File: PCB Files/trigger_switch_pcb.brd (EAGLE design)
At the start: 114 x 77.5 mm, 11 parts

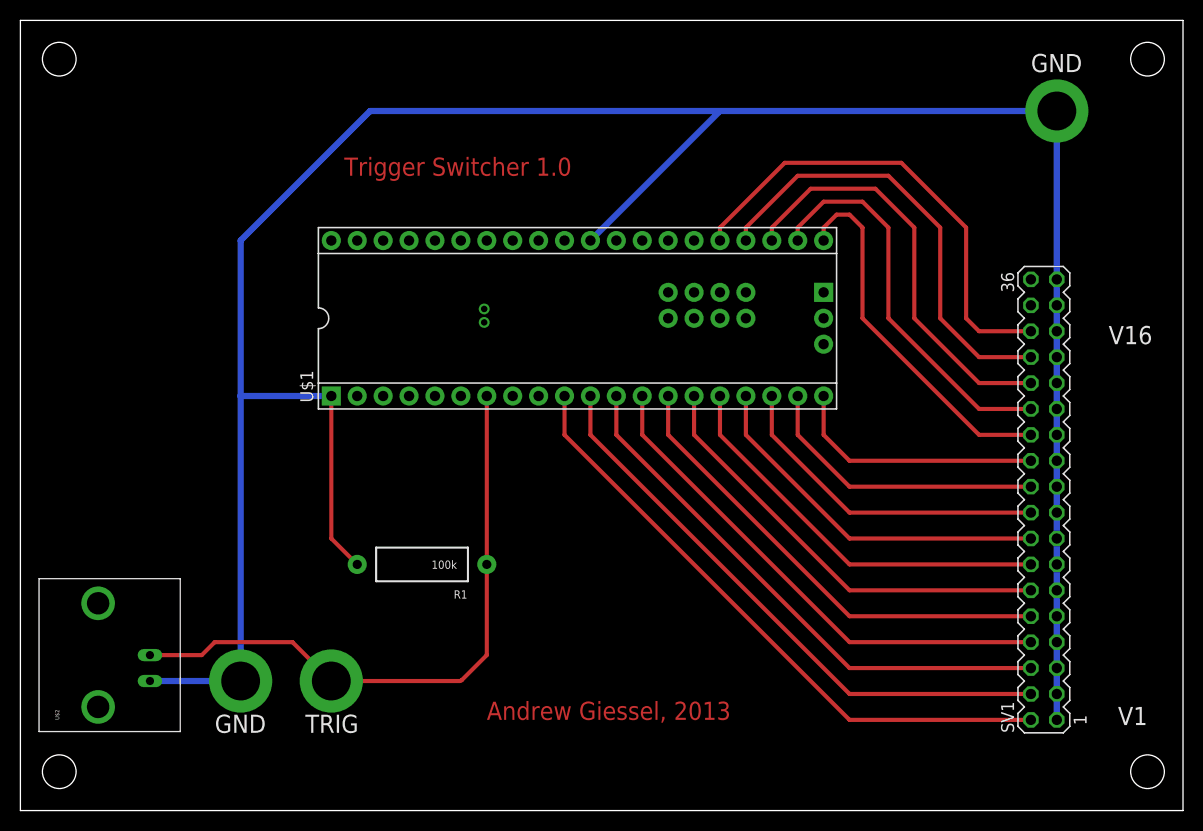
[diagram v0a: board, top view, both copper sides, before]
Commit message: SHRINK
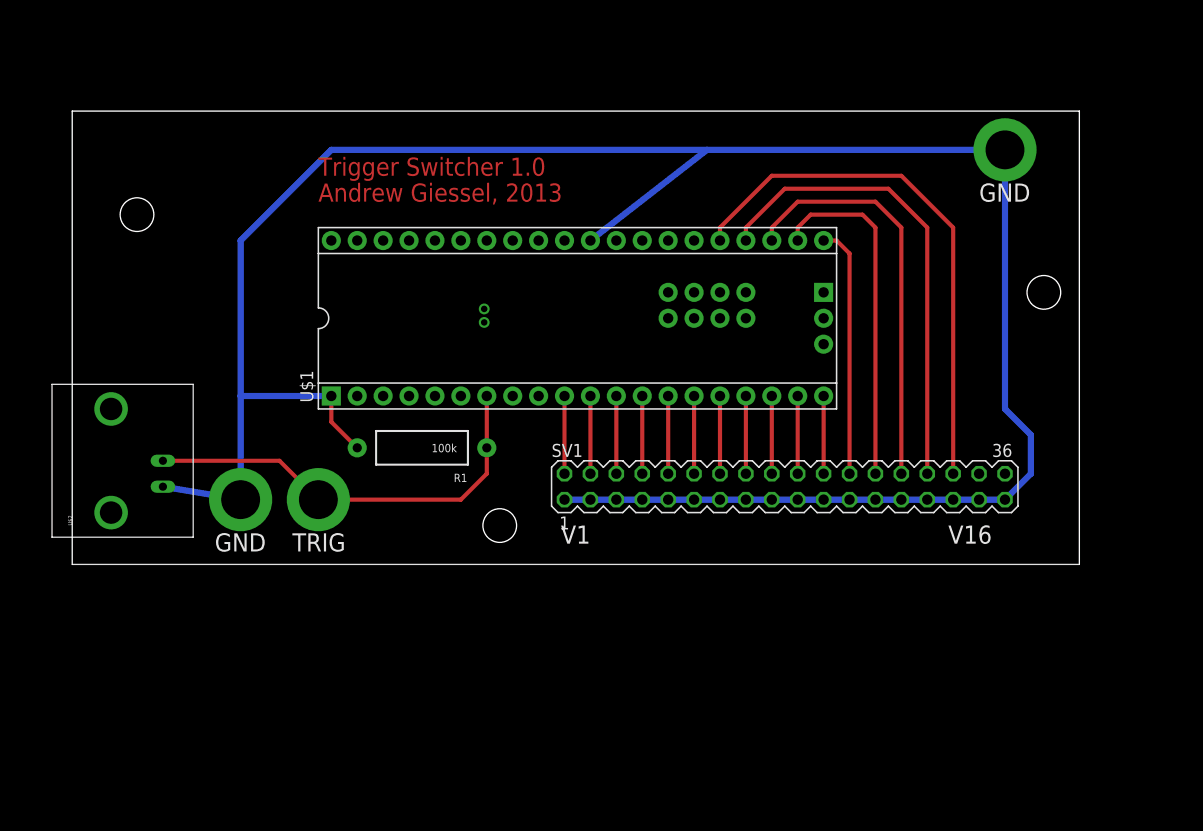
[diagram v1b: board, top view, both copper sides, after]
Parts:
- removed U$5: (no value), SparkFun-Electromechanical:STAND-OFF
- moved U$6 49.5 mm to (47.0, 39.4)
- moved SV1 25.4 mm to (74.9, 43.2), turned to 0 degrees
- moved U$4 25.0 mm to (100.3, 62.2)
- moved U$2 19.1 mm to (14.0, 45.7)
- moved JP2 17.8 mm to (29.2, 41.9)
- moved JP3 17.8 mm to (21.6, 41.9)
- moved U$3 17.0 mm to (11.4, 69.8)
- moved R1 11.4 mm to (39.4, 47.0)
- moved JP1 6.35 mm to (96.5, 76.2)
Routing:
- net V1: track 61.1 -> 7.62 mm
- net V2: track 57.5 -> 7.62 mm
- net V3: track 53.9 -> 7.62 mm
- net V4: track 50.3 -> 7.62 mm
- net V5: track 46.7 -> 7.62 mm
- net V6: track 43.1 -> 7.62 mm
- net V7: track 39.6 -> 7.62 mm
- net V8: track 36.0 -> 7.62 mm
- net V9: track 32.4 -> 7.62 mm
- net V10: track 28.8 -> 7.62 mm
- net GND: track 241.4 -> 220.8 mm
- net TRIG: track 61.6 -> 42.0 mm
- net V11: track 25.2 -> 7.62 mm
- net V12: track 36.3 -> 24.7 mm
- net V16: track 46.4 -> 52.5 mm
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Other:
- board size 114 x 77.5 mm -> 98.7 x 44.4 mm
